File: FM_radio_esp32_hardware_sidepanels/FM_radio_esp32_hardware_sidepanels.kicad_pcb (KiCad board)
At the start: 2 copper layers, 78 x 43 mm, 11 parts

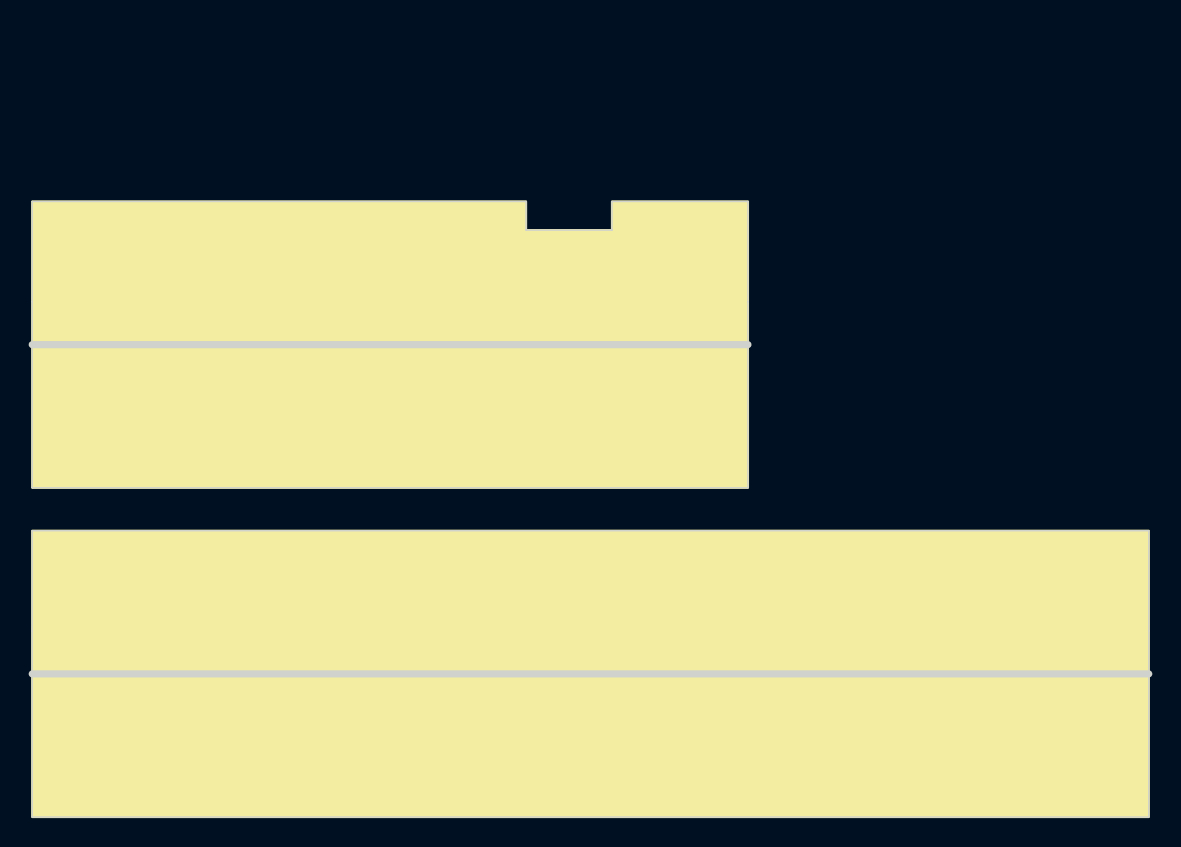
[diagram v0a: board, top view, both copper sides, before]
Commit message: side panels dimension update
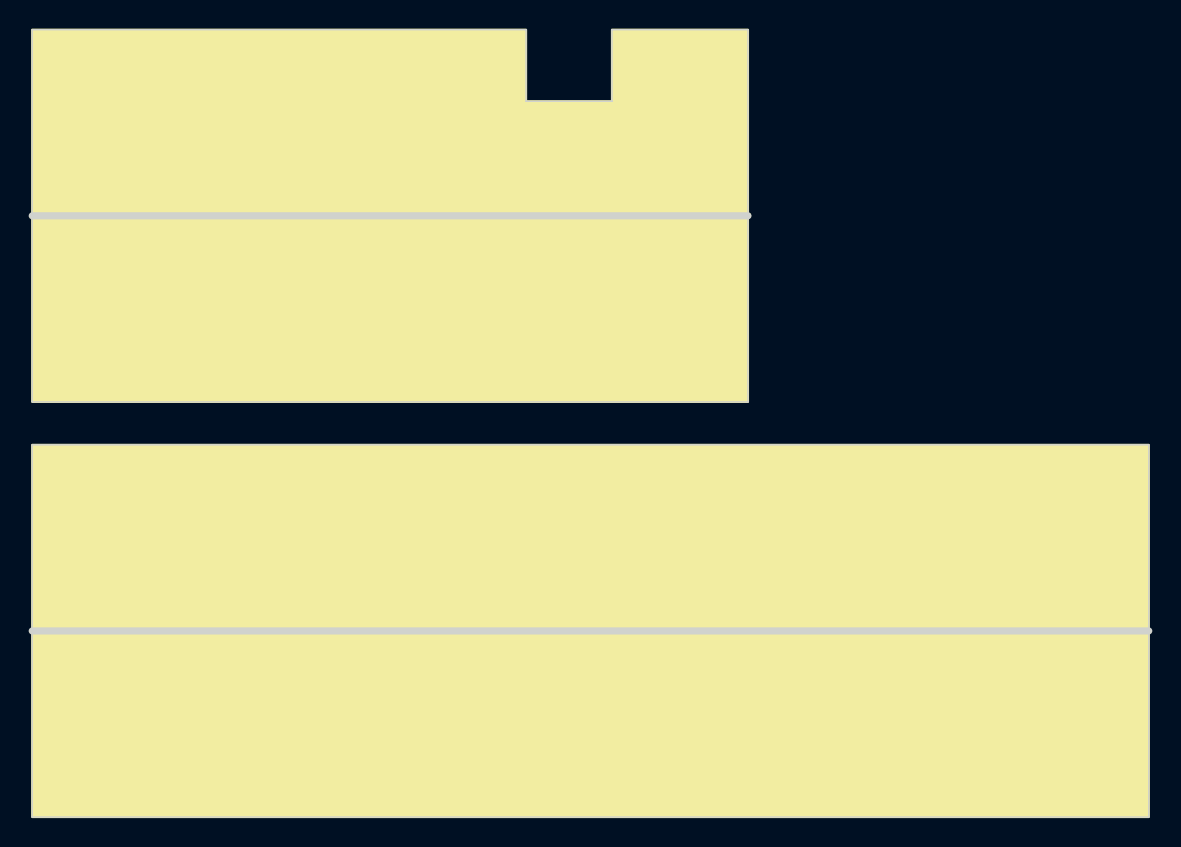
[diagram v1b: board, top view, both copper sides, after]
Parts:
- moved G*** 11.6 mm to (134.5, 103.0)
- moved H7 10.5 mm to (93.0, 81.5)
- moved H8 10.5 mm to (137.0, 81.5)
- moved H9 9.00 mm to (127.5, 84.5)
- moved TP1 9.00 mm to (117.0, 84.5)
- moved H5 7.50 mm to (93.0, 94.5)
- moved H6 7.50 mm to (137.0, 94.5)
- moved H3 4.50 mm to (93.0, 110.5)
- moved H4 4.50 mm to (165.0, 110.5)
- moved H1 1.50 mm to (93.0, 123.5)
- moved H2 1.50 mm to (165.0, 123.5)
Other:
- board size 78 x 43 mm -> 78 x 55 mm
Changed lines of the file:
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@@
   (net 1 "/ANT")
   (footprint "MountingHole:MountingHole_3.2mm_M3" (layer "F.Cu")
-    (at 165 125)
+    (at 165 123.5)
     (descr "Mounting Hole 3.2mm, no annular, M3")
     (tags "mounting hole 3.2mm no annular m3")
@@
   )
   (footprint "MountingHole:MountingHole_3.2mm_M3" (layer "F.Cu")
-    (at 93 102)
+    (at 93 94.5)
     (descr "Mounting Hole 3.2mm, no annular, M3")
     (tags "mounting hole 3.2mm no annular m3")
@@
   )
   (footprint "MountingHole:MountingHole_3.2mm_M3" (layer "F.Cu")
-    (at 137 102)
+    (at 137 94.5)
     (descr "Mounting Hole 3.2mm, no annular, M3")
     (tags "mounting hole 3.2mm no annular m3")
@@
   )
   (footprint "MountingHole:MountingHole_3.2mm_M3" (layer "F.Cu")
-    (at 93 115)
+    (at 93 110.5)
     (descr "Mounting Hole 3.2mm, no annular, M3")
     (tags "mounting hole 3.2mm no annular m3")
@@
   )
   (footprint "MountingHole:MountingHole_3.2mm_M3" (layer "F.Cu")
-    (at 137 92)
+    (at 137 81.5)
     (descr "Mounting Hole 3.2mm, no annular, M3")
     (tags "mounting hole 3.2mm no annular m3")
@@
   )
   (footprint "MountingHole:MountingHole_3.2mm_M3" (layer "F.Cu")
-    (at 165 115)
+    (at 165 110.5)
     (descr "Mounting Hole 3.2mm, no annular, M3")
     (tags "mounting hole 3.2mm no annular m3")
@@
   )
   (footprint "MountingHole:MountingHole_3.2mm_M3_DIN965_Pad" (layer "F.Cu")
-    (at 127.5 93.5)
+    (at 127.5 84.5)
     (descr "Mounting Hole 3.2mm, M3, DIN965")
     (tags "mounting hole 3.2mm m3 din965")
@@
   )
   (footprint "MountingHole:MountingHole_3.2mm_M3" (layer "F.Cu")
-    (at 93 92)
+    (at 93 81.5)
     (descr "Mounting Hole 3.2mm, no annular, M3")
     (tags "mounting hole 3.2mm no annular m3")
@@
   )
   (footprint "MountingHole:MountingHole_3.2mm_M3" (layer "F.Cu")
-    (at 93 125)
+    (at 93 123.5)
     (descr "Mounting Hole 3.2mm, no annular, M3")
     (tags "mounting hole 3.2mm no annular m3")
@@
   )
   (footprint "TestPoint:TestPoint_Keystone_5019_Minature" (layer "B.Cu")
-    (at 117 93.5 180)
+    (at 117 84.5 180)
     (descr "SMT Test Point- Micro Miniature 5019, http://www.keyelco.com/product-pdf.cfm?p=1357")
     (tags "Test Point")
@@
   )
   (footprint "_local_Library:electronics_fig_4" (layer "B.Cu")
-    (at 129.5 113.5 180)
+    (at 134.5 103 180)
     (attr board_only exclude_from_pos_files exclude_from_bom)
     (fp_text reference "G***" (at 0 0) (layer "B.SilkS") hide
@@
       ) (layer "B.SilkS") (width 0) (fill solid))
   )
-  (gr_rect (start 168 110) (end 90 130) (layer "F.SilkS") (width 0.15) (fill solid))
+  (gr_rect (start 168 104) (end 90 130) (layer "F.SilkS") (width 0.15) (fill solid))
   (gr_poly
     (pts
-      (xy 124.5 89)
-      (xy 130.5 89)
-      (xy 130.5 87)
-      (xy 140 87)
-      (xy 140 107)
-      (xy 90 107)
-      (xy 90 87)
-      (xy 124.5 87)
+      (xy 124.5 80)
+      (xy 130.5 80)
+      (xy 130.5 75)
+      (xy 140 75)
+      (xy 140 101)
+      (xy 90 101)
+      (xy 90 75)
+      (xy 124.5 75)
     ) (layer "F.SilkS") (width 0.15) (fill solid))
-  (gr_line (start 90 97) (end 140 97) (layer "Edge.Cuts") (width 0.5))
-  (gr_line (start 90 117) (end 90 110) (layer "Edge.Cuts") (width 0.1))
-  (gr_line (start 124.5 89) (end 124.5 87) (layer "Edge.Cuts") (width 0.1))
-  (gr_line (start 168 110) (end 168 117) (layer "Edge.Cuts") (width 0.1))
-  (gr_line (start 140 87) (end 130.5 87) (layer "Edge.Cuts") (width 0.1))
+  (gr_line (start 90 88) (end 140 88) (layer "Edge.Cuts") (width 0.5))
+  (gr_line (start 90 117) (end 90 104) (layer "Edge.Cuts") (width 0.1))
+  (gr_line (start 124.5 80) (end 124.5 75) (layer "Edge.Cuts") (width 0.1))
+  (gr_line (start 168 104) (end 168 117) (layer "Edge.Cuts") (width 0.1))
+  (gr_line (start 140 75) (end 130.5 75) (layer "Edge.Cuts") (width 0.1))
   (gr_line (start 168 130) (end 90 130) (layer "Edge.Cuts") (width 0.1))
-  (gr_line (start 140 87) (end 140 94) (layer "Edge.Cuts") (width 0.1))
-  (gr_line (start 140 107) (end 90 107) (layer "Edge.Cuts") (width 0.1))
-  (gr_line (start 140 94) (end 140 107) (layer "Edge.Cuts") (width 0.1))
-  (gr_line (start 90 107) (end 90 94) (layer "Edge.Cuts") (width 0.1))
-  (gr_line (start 124.5 87) (end 90 87) (layer "Edge.Cuts") (width 0.1))
-  (gr_line (start 130.5 89) (end 124.5 89) (layer "Edge.Cuts") (width 0.1))
-  (gr_line (start 90 94) (end 90 87) (layer "Edge.Cuts") (width 0.1))
+  (gr_line (start 140 75) (end 140 88) (layer "Edge.Cuts") (width 0.1))
+  (gr_line (start 140 101) (end 90 101) (layer "Edge.Cuts") (width 0.1))
+  (gr_line (start 140 88) (end 140 101) (layer "Edge.Cuts") (width 0.1))
+  (gr_line (start 90 101) (end 90 88) (layer "Edge.Cuts") (width 0.1))
+  (gr_line (start 124.5 75) (end 90 75) (layer "Edge.Cuts") (width 0.1))
+  (gr_line (start 130.5 80) (end 124.5 80) (layer "Edge.Cuts") (width 0.1))
+  (gr_line (start 90 88) (end 90 75) (layer "Edge.Cuts") (width 0.1))
   (gr_line (start 168 117) (end 168 130) (layer "Edge.Cuts") (width 0.1))
-  (gr_line (start 90 120) (end 168 120) (layer "Edge.Cuts") (width 0.5))
+  (gr_line (start 90 117) (end 168 117) (layer "Edge.Cuts") (width 0.5))
   (gr_line (start 90 130) (end 90 117) (layer "Edge.Cuts") (width 0.1))
-  (gr_line (start 90 110) (end 168 110) (layer "Edge.Cuts") (width 0.1))
-  (gr_line (start 130.5 87) (end 130.5 89) (layer "Edge.Cuts") (width 0.1))
+  (gr_line (start 90 104) (end 168 104) (layer "Edge.Cuts") (width 0.1))
+  (gr_line (start 130.5 75) (end 130.5 80) (layer "Edge.Cuts") (width 0.1))
   (dimension (type aligned) (layer "Dwgs.User")
-    (pts (xy 127.5 93.5) (xy 140 93.5))
-    (height -9)
-    (gr_text "12.5000 mm" (at 133.75 83.35) (layer "Dwgs.User")
+    (pts (xy 160.5 130) (xy 160.5 117))
+    (height 16.5)
+    (gr_text "13.0000 mm" (at 175.85 123.5 90) (layer "Dwgs.User")
       (effects (font (size 1 1) (thickness 0.15)))
     )
     (format (units 3) (units_format 1) (precision 4))
-    (style (thickness 0.1) (arrow_length 1.27) (text_position_mode 0) (extension_height 0.58642) (extension_offset 0.5) keep_text_aligned)
+    (style (thickness 0.15) (arrow_length 1.27) (text_position_mode 0) (extension_height 0.58642) (extension_offset 0.5) keep_text_aligned)
+  )
+  (dimension (type aligned) (layer "Dwgs.User")
+    (pts (xy 90 130) (xy 168 130))
+    (height 10.499999)
+    (gr_text "78.0000 mm" (at 129 139.349999) (layer "Dwgs.User")
+      (effects (font (size 1 1) (thickness 0.15)))
+    )
+    (format (units 3) (units_format 1) (precision 4))
+    (style (thickness 0.15) (arrow_length 1.27) (text_position_mode 0) (extension_height 0.58642) (extension_offset 0.5) keep_text_aligned)
   )
   (dimension (type aligned) (layer "Dwgs.User")
@@
   )
   (dimension (type aligned) (layer "Dwgs.User")
-    (pts (xy 127.5 93.5) (xy 127.5 97))
-    (height -15.5)
-    (gr_text "3.5000 mm" (at 141.85 95.25 90) (layer "Dwgs.User")
+    (pts (xy 127.5 84.5) (xy 140 84.5))
+    (height -16)
+    (gr_text "12.5000 mm" (at 133.75 67.35) (layer "Dwgs.User")
       (effects (font (size 1 1) (thickness 0.15)))
     )
     (format (units 3) (units_format 1) (precision 4))
-    (style (thickness 0.1) (arrow_length 1.27) (text_position_mode 0) (extension_height 0.58642) (extension_offset 0.5) keep_text_aligned)
+    (style (thickness 0.15) (arrow_length 1.27) (text_position_mode 0) (extension_height 0.58642) (extension_offset 0.5) keep_text_aligned)
+  )
+  (dimension (type aligned) (layer "Dwgs.User")
+    (pts (xy 90 75) (xy 140 75))
+    (height -12.5)
+    (gr_text "50.0000 mm" (at 115 61.35) (layer "Dwgs.User")
+      (effects (font (size 1 1) (thickness 0.15)))
+    )
+    (format (units 3) (units_format 1) (precision 4))
+    (style (thickness 0.15) (arrow_length 1.27) (text_position_mode 0) (extension_height 0.58642) (extension_offset 0.5) keep_text_aligned)
   )
   (target plus (at 90 130) (size 5) (width 0.1) (layer "Edge.Cuts"))
-  (segment (start 117 93.5) (end 127.5 93.5) (width 0.8) (layer "B.Cu") (net 1))
+  (segment (start 117 84.5) (end 127.5 84.5) (width 0.8) (layer "B.Cu") (net 1))
 )
